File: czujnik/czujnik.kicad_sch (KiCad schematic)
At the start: 9 parts, among them J4 Conn_01x08, J5 Conn_01x10, U5 BME280, U6 MB85RS256B

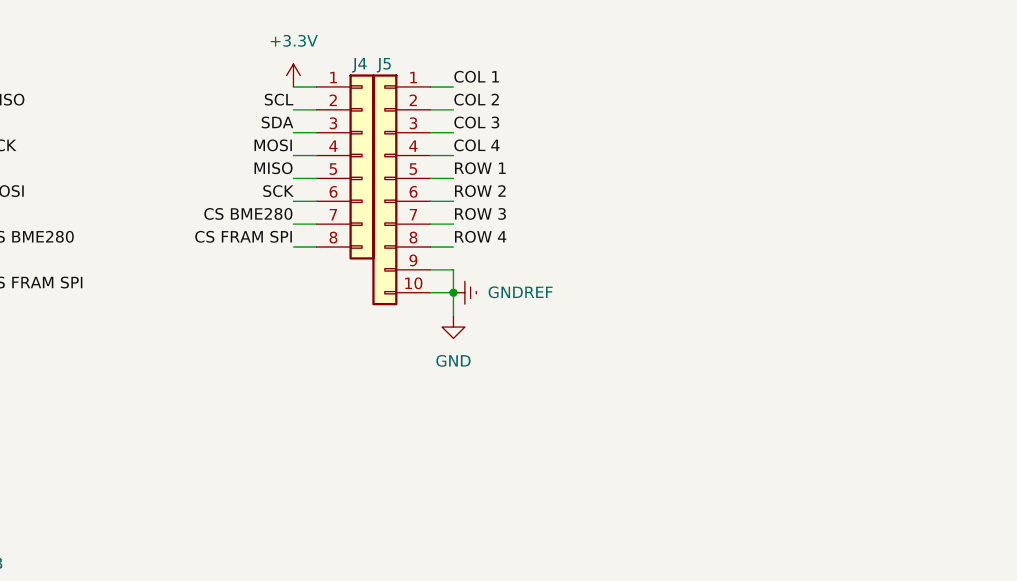
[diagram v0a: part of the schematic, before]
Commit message: Zmianakonnektora
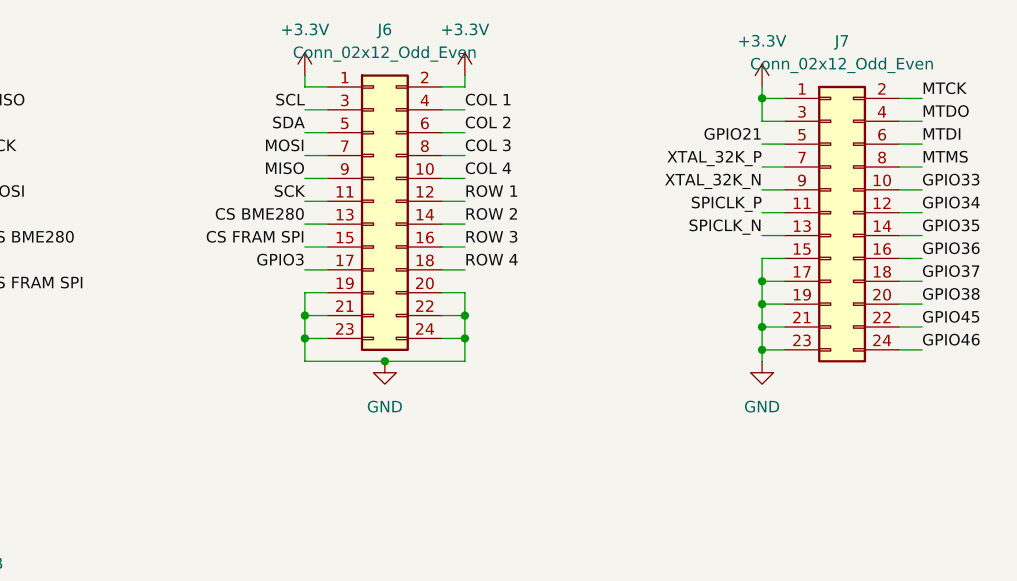
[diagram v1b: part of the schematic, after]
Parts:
- removed J4: Conn_01x08, Connector_PinHeader_2.54mm:PinHeader_1x08_P2.54mm_Vertical, symbol Connector_Generic:Conn_01x08
- removed J5: Conn_01x10, Connector_PinHeader_2.54mm:PinHeader_1x10_P2.54mm_Vertical, symbol Connector_Generic:Conn_01x10
- added J6, J7: Conn_02x12_Odd_Even, Connector_PinSocket_2.54mm:PinSocket_2x12_P2.54mm_Vertical, symbol Connector_Generic:Conn_02x12_Odd_Even
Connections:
- net +3.3V: now also J6.1 (Pin_1), J6.2 (Pin_2), J7.1 (Pin_1), J7.3 (Pin_3)
- net COL 1: now also J6.4 (Pin_4)
- net COL 2: now also J6.6 (Pin_6)
- net COL 3: now also J6.8 (Pin_8)
- net COL 4: now also J6.10 (Pin_10)
- net CS BME280: now also J6.13 (Pin_13)
- net CS FRAM SPI: now also J6.15 (Pin_15)
- net GND: now also J6.19 (Pin_19), J6.20 (Pin_20), J6.21 (Pin_21), J6.22 (Pin_22), J6.23 (Pin_23), J6.24 (Pin_24), J7.15 (Pin_15), J7.17 (Pin_17), J7.19 (Pin_19), J7.21 (Pin_21), J7.23 (Pin_23)
- net MISO: now also J6.9 (Pin_9)
- net MOSI: now also J6.7 (Pin_7)
- net ROW 1: now also J6.12 (Pin_12)
- net ROW 2: now also J6.14 (Pin_14)
- net ROW 3: now also J6.16 (Pin_16)
- net ROW 4: now also J6.18 (Pin_18)
- net SCK: now also J6.11 (Pin_11)
- net SCL: now also J6.3 (Pin_3)
- net SDA: now also J6.5 (Pin_5)
- new net GPIO21: J7.5 (Pin_5)
- new net GPIO3: J6.17 (Pin_17)
- new net GPIO33: J7.10 (Pin_10)
- new net GPIO34: J7.12 (Pin_12)
- new net GPIO35: J7.14 (Pin_14)
- new net GPIO36: J7.16 (Pin_16)
- new net GPIO37: J7.18 (Pin_18)
- new net GPIO38: J7.20 (Pin_20)
- new net GPIO45: J7.22 (Pin_22)
- new net GPIO46: J7.24 (Pin_24)
- new net MTCK: J7.2 (Pin_2)
- new net MTDI: J7.6 (Pin_6)
- new net MTDO: J7.4 (Pin_4)
- new net MTMS: J7.8 (Pin_8)
- new net SPICLK_N: J7.13 (Pin_13)
- new net SPICLK_P: J7.11 (Pin_11)
- new net XTAL_32K_N: J7.9 (Pin_9)
- new net XTAL_32K_P: J7.7 (Pin_7)

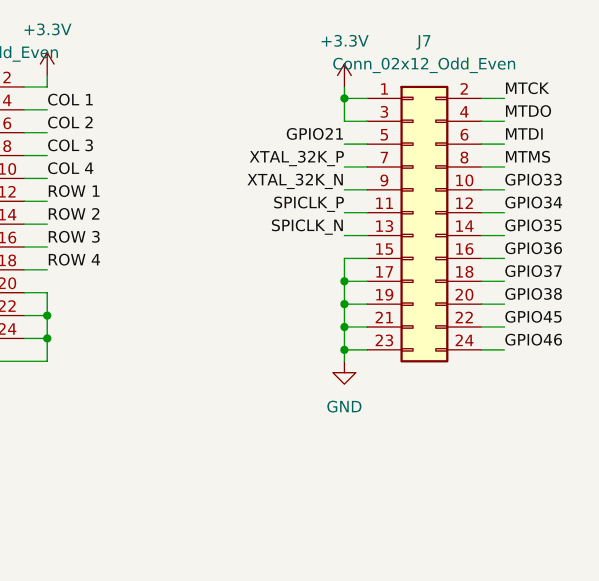
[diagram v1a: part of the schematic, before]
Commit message: Zmianakonnektorav2
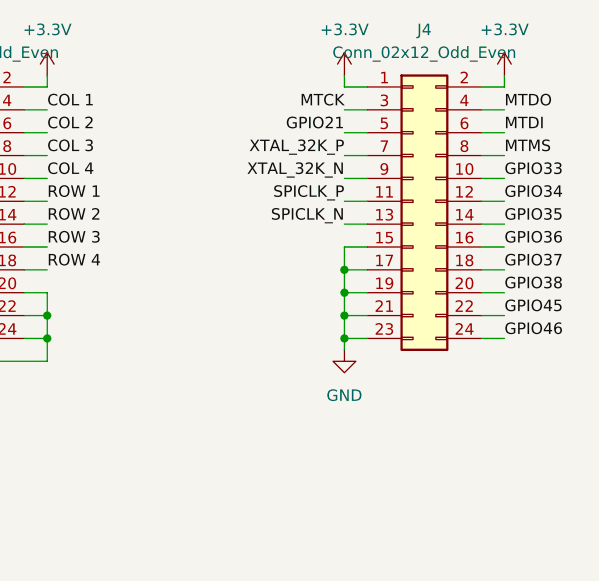
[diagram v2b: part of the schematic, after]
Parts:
- removed J7: Conn_02x12_Odd_Even, Connector_PinSocket_2.54mm:PinSocket_2x12_P2.54mm_Vertical, symbol Connector_Generic:Conn_02x12_Odd_Even
- added J4: Conn_02x12_Odd_Even, Connector_PinSocket_2.54mm:PinSocket_2x12_P2.54mm_Vertical, symbol Connector_Generic:Conn_02x12_Odd_Even
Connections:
- net +3.3V: now also J4.1 (Pin_1), J4.2 (Pin_2)
- net GND: now also J4.15 (Pin_15), J4.17 (Pin_17), J4.19 (Pin_19), J4.21 (Pin_21), J4.23 (Pin_23)
- net GPIO21: now also J4.5 (Pin_5)
- net GPIO33: now also J4.10 (Pin_10)
- net GPIO34: now also J4.12 (Pin_12)
- net GPIO35: now also J4.14 (Pin_14)
- net GPIO36: now also J4.16 (Pin_16)
- net GPIO37: now also J4.18 (Pin_18)
- net GPIO38: now also J4.20 (Pin_20)
- net GPIO45: now also J4.22 (Pin_22)
- net GPIO46: now also J4.24 (Pin_24)
- net MTCK: now also J4.3 (Pin_3)
- net MTDI: now also J4.6 (Pin_6)
- net MTDO: now also J4.4 (Pin_4)
- net MTMS: now also J4.8 (Pin_8)
- net SPICLK_N: now also J4.13 (Pin_13)
- net SPICLK_P: now also J4.11 (Pin_11)
- net XTAL_32K_N: now also J4.9 (Pin_9)
- net XTAL_32K_P: now also J4.7 (Pin_7)
